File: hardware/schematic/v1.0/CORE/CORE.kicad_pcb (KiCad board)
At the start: 4 copper layers, 0 parts

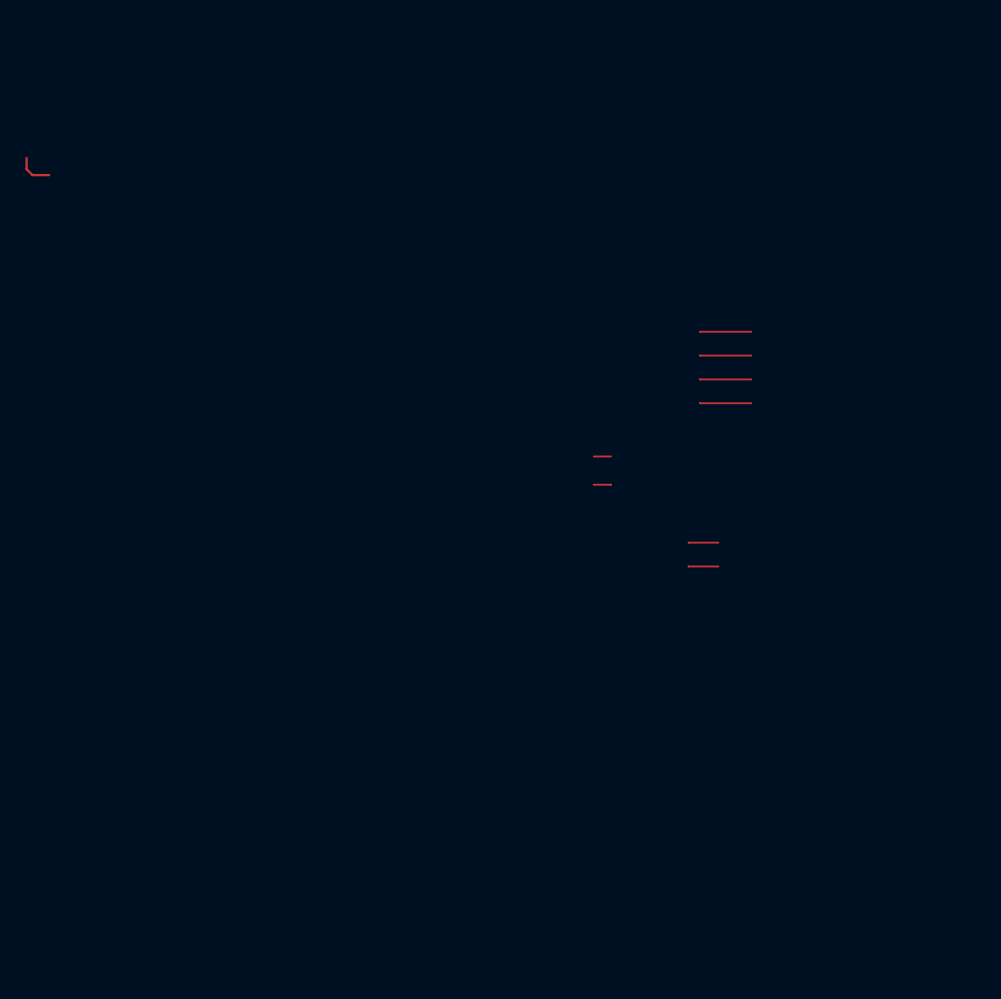
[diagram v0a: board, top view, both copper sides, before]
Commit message: sch and pcb update
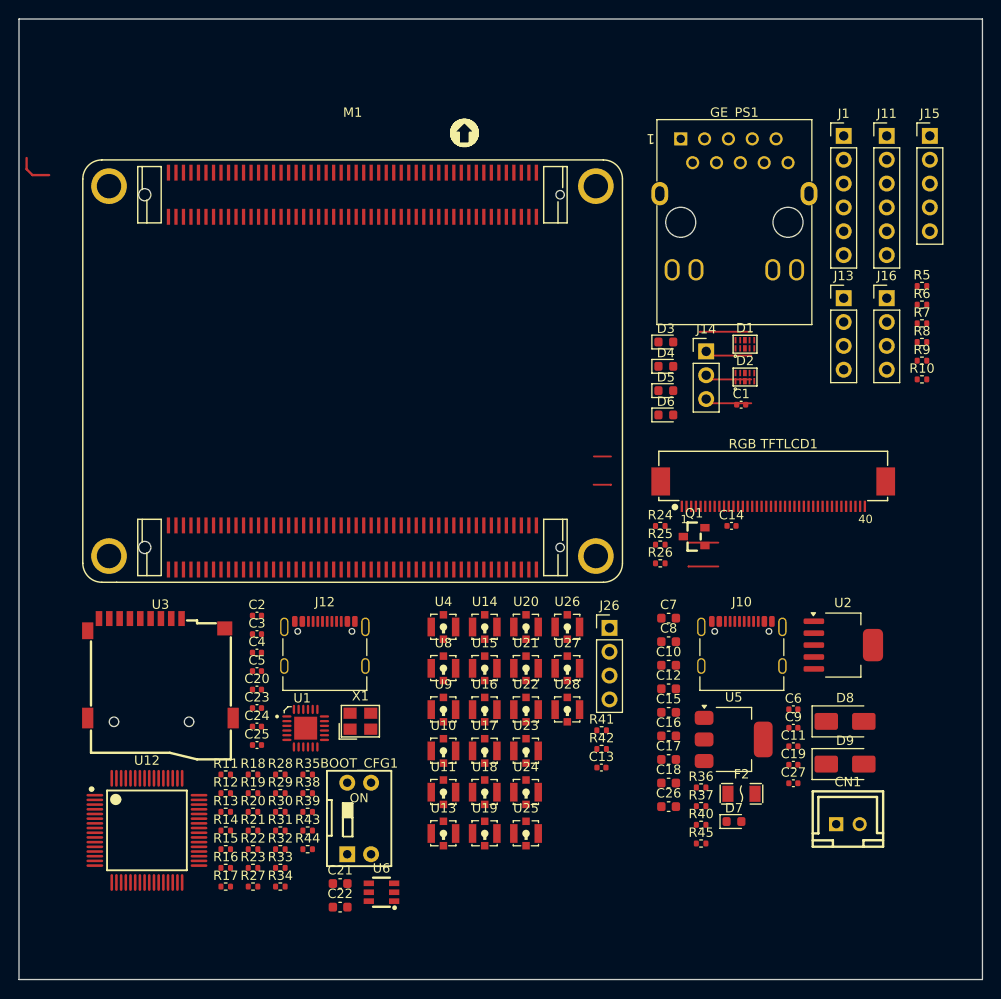
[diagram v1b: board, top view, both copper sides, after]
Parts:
- added BOOT_CFG1: CSW-2P, Counter:CSW DIP-2P, F.Cu at (140.1, 137.9)
- added C1: 100nF, Capacitor_SMD:C_0402_1005Metric, F.Cu at (182.1, 90.0)
- added C10: 10uF, Capacitor_SMD:C_0603_1608Metric, F.Cu at (174.4, 117.7)
- added C11: 100nF, Capacitor_SMD:C_0402_1005Metric, F.Cu at (187.6, 126.4)
- added C12: 10uF, Capacitor_SMD:C_0603_1608Metric, F.Cu at (174.4, 120.3)
- added C13: 1nF, Capacitor_SMD:C_0402_1005Metric, F.Cu at (167.2, 128.6)
- added C14: 100nF, Capacitor_SMD:C_0402_1005Metric, F.Cu at (181.1, 102.9)
- added C15: 10uF, Capacitor_SMD:C_0603_1608Metric, F.Cu at (174.4, 122.8)
- added C16: 100nF, Capacitor_SMD:C_0603_1608Metric, F.Cu at (174.4, 125.3)
- added C17: 10uF, Capacitor_SMD:C_0603_1608Metric, F.Cu at (174.4, 127.8)
- added C18: 100nF, Capacitor_SMD:C_0603_1608Metric, F.Cu at (174.4, 130.3)
- added C19: 100nF, Capacitor_SMD:C_0402_1005Metric, F.Cu at (187.6, 128.3)
- added C2: 100nF, Capacitor_SMD:C_0402_1005Metric, F.Cu at (130.5, 112.5)
- added C20: 100nF, Capacitor_SMD:C_0402_1005Metric, F.Cu at (130.5, 120.3)
- added C21: 10uF, Capacitor_SMD:C_0603_1608Metric, F.Cu at (139.4, 141.0)
- added C22: 10uF, Capacitor_SMD:C_0603_1608Metric, F.Cu at (139.4, 143.5)
- added C23: 100nF, Capacitor_SMD:C_0402_1005Metric, F.Cu at (130.5, 122.3)
- added C24: 30pF, Capacitor_SMD:C_0402_1005Metric, F.Cu at (130.5, 124.3)
- added C25: 30pF, Capacitor_SMD:C_0402_1005Metric, F.Cu at (130.5, 126.2)
- added C26: 10uF, Capacitor_SMD:C_0603_1608Metric, F.Cu at (174.4, 132.8)
- added C27: 100nF, Capacitor_SMD:C_0402_1005Metric, F.Cu at (187.6, 130.3)
- added C3: 100nF, Capacitor_SMD:C_0402_1005Metric, F.Cu at (130.5, 114.4)
- added C4: 10uF, Capacitor_SMD:C_0402_1005Metric, F.Cu at (130.5, 116.4)
- added C5: 100nF, Capacitor_SMD:C_0402_1005Metric, F.Cu at (130.5, 118.4)
- added C6: 100nF, Capacitor_SMD:C_0402_1005Metric, F.Cu at (187.6, 122.4)
- added C7: 10uF, Capacitor_SMD:C_0603_1608Metric, F.Cu at (174.4, 112.7)
- added C8: 10uF, Capacitor_SMD:C_0603_1608Metric, F.Cu at (174.4, 115.2)
- added C9: 10nF, Capacitor_SMD:C_0402_1005Metric, F.Cu at (187.6, 124.4)
- added CN1: LAIL-PHC2_54-2P-01-XH-L, JLCImport:LAIL-PHC2_54-2P-01-XH-L, F.Cu at (193.5, 134.7)
- added D1: AZ1143-04F.R7G, Counter:DFN2510P10E, F.Cu at (181.4, 84.8)
- added D2: AZ1143-04F.R7G, Counter:DFN2510P10E, F.Cu at (181.4, 88.3)
- added D3: LED, LED_SMD:LED_0603_1608Metric, F.Cu at (174.1, 83.3)
- added D4: LED, LED_SMD:LED_0603_1608Metric, F.Cu at (174.1, 85.9)
- added D5: LED, LED_SMD:LED_0603_1608Metric, F.Cu at (174.1, 88.5)
- added D6: LED, LED_SMD:LED_0603_1608Metric, F.Cu at (174.1, 91.1)
- added D7: LED, LED_SMD:LED_0603_1608Metric, F.Cu at (181.3, 134.4)
- added D8: SS34, Diode_SMD:D_SMA, F.Cu at (193.2, 123.7)
- added D9: SS34, Diode_SMD:D_SMA, F.Cu at (193.2, 128.3)
- added F2: BSMD1206C-1300T, JLCImport:BSMD1206C-1300T, F.Cu at (182.1, 131.4)
- added GE_PS1: HR911131A, Counter:HR911131A, F.Cu at (175.6, 61.7)
- added J1: Conn_01x06_Socket, Connector_PinHeader_2.54mm:PinHeader_1x06_P2.54mm_Vertical, F.Cu at (193.0, 61.3)
- added J10: USB_C_Receptacle_USB2.0_16P, Connector_USB:USB_C_Receptacle_Palconn_UTC16-G, F.Cu at (182.2, 115.6)
- added J11: Conn_01x06_Socket, Connector_PinHeader_2.54mm:PinHeader_1x06_P2.54mm_Vertical, F.Cu at (197.6, 61.3)
- added J12: USB_C_Receptacle_USB2.0_16P, Connector_USB:USB_C_Receptacle_Palconn_UTC16-G, F.Cu at (137.7, 115.6)
- added J13: Conn_01x04_Socket, Connector_PinHeader_2.54mm:PinHeader_1x04_P2.54mm_Vertical, F.Cu at (193.0, 78.6)
- added J14: Conn_01x03_Socket, Connector_PinHeader_2.54mm:PinHeader_1x03_P2.54mm_Vertical, F.Cu at (178.4, 84.3)
- added J15: Conn_01x05_Socket, Connector_PinHeader_2.54mm:PinHeader_1x05_P2.54mm_Vertical, F.Cu at (202.2, 61.3)
- added J16: Conn_01x04_Socket, Connector_PinHeader_2.54mm:PinHeader_1x04_P2.54mm_Vertical, F.Cu at (197.6, 78.6)
- added J26: Conn_01x04_Socket, Connector_PinHeader_2.54mm:PinHeader_1x04_P2.54mm_Vertical, F.Cu at (168.1, 113.8)
- added M1: ZYNQ7010&7020, Counter:ZYNQ7010&7020_CB, F.Cu at (126.3, 102.8)
- added Q1: Si2302CDS-T1-GE3, JLCImport:Si2302CDS-T1-GE3, F.Cu at (177.1, 104.0)
- added R10: 499R, Resistor_SMD:R_0402_1005Metric, F.Cu at (201.3, 87.3)
- added R11: 20K, Resistor_SMD:R_0402_1005Metric, F.Cu at (127.2, 129.4)
- added R12: 20K, Resistor_SMD:R_0402_1005Metric, F.Cu at (127.2, 131.4)
- added R13: 10K, Resistor_SMD:R_0402_1005Metric, F.Cu at (127.2, 133.4)
- added R14: 10K, Resistor_SMD:R_0402_1005Metric, F.Cu at (127.2, 135.4)
- added R15: 4.7K, Resistor_SMD:R_0402_1005Metric, F.Cu at (127.2, 137.3)
- added R16: 330, Resistor_SMD:R_0402_1005Metric, F.Cu at (127.2, 139.3)
- added R17: 0, Resistor_SMD:R_0402_1005Metric, F.Cu at (127.2, 141.3)
- added R18: 10K, Resistor_SMD:R_0402_1005Metric, F.Cu at (130.1, 129.4)
- added R19: 4.7K, Resistor_SMD:R_0402_1005Metric, F.Cu at (130.1, 131.4)
- added R20: 4.7K, Resistor_SMD:R_0402_1005Metric, F.Cu at (130.1, 133.4)
- added R21: 4.7K, Resistor_SMD:R_0402_1005Metric, F.Cu at (130.1, 135.4)
- added R22: 4.7K, Resistor_SMD:R_0402_1005Metric, F.Cu at (130.1, 137.3)
- added R23: 4.7K, Resistor_SMD:R_0402_1005Metric, F.Cu at (130.1, 139.3)
- added R24: 10K, Resistor_SMD:R_0402_1005Metric, F.Cu at (173.5, 102.9)
- added R25: 1K, Resistor_SMD:R_0402_1005Metric, F.Cu at (173.5, 104.9)
- added R26: 10, Resistor_SMD:R_0402_1005Metric, F.Cu at (173.5, 106.9)
- added R27: 10R, Resistor_SMD:R_0402_1005Metric, F.Cu at (130.1, 141.3)
- added R28: 10R, Resistor_SMD:R_0402_1005Metric, F.Cu at (133.0, 129.4)
- added R29: 33R, Resistor_SMD:R_0402_1005Metric, F.Cu at (133.0, 131.4)
- added R30: 33R, Resistor_SMD:R_0402_1005Metric, F.Cu at (133.0, 133.4)
- added R31: 33R, Resistor_SMD:R_0402_1005Metric, F.Cu at (133.0, 135.4)
- added R32: 33R, Resistor_SMD:R_0402_1005Metric, F.Cu at (133.0, 137.3)
- added R33: 2K, Resistor_SMD:R_0402_1005Metric, F.Cu at (133.0, 139.3)
- added R34: 10K, Resistor_SMD:R_0402_1005Metric, F.Cu at (133.0, 141.3)
- added R35: 12K/%1, Resistor_SMD:R_0402_1005Metric, F.Cu at (135.9, 129.4)
- added R36: 5.1K, Resistor_SMD:R_0402_1005Metric, F.Cu at (177.8, 130.8)
- added R37: 5.1K, Resistor_SMD:R_0402_1005Metric, F.Cu at (177.8, 132.8)
- added R38: 5.1K, Resistor_SMD:R_0402_1005Metric, F.Cu at (135.9, 131.4)
- added R39: 5.1K, Resistor_SMD:R_0402_1005Metric, F.Cu at (135.9, 133.4)
- added R40: 0, Resistor_SMD:R_0402_1005Metric, F.Cu at (177.8, 134.7)
- added R41: 49.9, Resistor_SMD:R_0402_1005Metric, F.Cu at (167.2, 124.7)
- added R42: 49.9, Resistor_SMD:R_0402_1005Metric, F.Cu at (167.2, 126.7)
- added R43: 0, Resistor_SMD:R_0402_1005Metric, F.Cu at (135.9, 135.4)
- added R44: 0, Resistor_SMD:R_0402_1005Metric, F.Cu at (135.9, 137.3)
- added R45: 1K, Resistor_SMD:R_0402_1005Metric, F.Cu at (177.8, 136.7)
- added R5: 499R, Resistor_SMD:R_0402_1005Metric, F.Cu at (201.3, 77.3)
- added R6: 499R, Resistor_SMD:R_0402_1005Metric, F.Cu at (201.3, 79.3)
- added R7: 499R, Resistor_SMD:R_0402_1005Metric, F.Cu at (201.3, 81.3)
- added R8: 499R, Resistor_SMD:R_0402_1005Metric, F.Cu at (201.3, 83.3)
- added R9: 499R, Resistor_SMD:R_0402_1005Metric, F.Cu at (201.3, 85.3)
- added RGB TFTLCD1: RGBLCD, AD:FPC-TOP40, F.Cu at (175.8, 100.9)
- added U1: TXS02612RTWR, Counter:QFN24_RTW, F.Cu at (135.7, 124.4)
- added U10: IPEX1, Counter:JLC_IPEX-1, F.Cu at (150.4, 126.9)
- added U11: IPEX1, Counter:JLC_IPEX-1, F.Cu at (150.4, 131.3)
- added U12: FT2232HL, JLCImport:FT2232HL, F.Cu at (118.8, 135.3)
- added U13: IPEX1, Counter:JLC_IPEX-1, F.Cu at (150.4, 135.7)
- added U14: IPEX1, Counter:JLC_IPEX-1, F.Cu at (154.8, 113.7)
- added U15: IPEX1, Counter:JLC_IPEX-1, F.Cu at (154.8, 118.1)
- added U16: IPEX1, Counter:JLC_IPEX-1, F.Cu at (154.8, 122.5)
- added U17: IPEX1, Counter:JLC_IPEX-1, F.Cu at (154.8, 126.9)
- added U18: IPEX1, Counter:JLC_IPEX-1, F.Cu at (154.8, 131.3)
- added U19: IPEX1, Counter:JLC_IPEX-1, F.Cu at (154.8, 135.7)
- added U2: TPS78633, Package_TO_SOT_SMD:SOT-223-6, F.Cu at (193.0, 115.6)
- added U20: IPEX1, Counter:JLC_IPEX-1, F.Cu at (159.2, 113.7)
- added U21: IPEX1, Counter:JLC_IPEX-1, F.Cu at (159.2, 118.1)
- added U22: IPEX1, Counter:JLC_IPEX-1, F.Cu at (159.2, 122.5)
- added U23: IPEX1, Counter:JLC_IPEX-1, F.Cu at (159.2, 126.9)
- added U24: IPEX1, Counter:JLC_IPEX-1, F.Cu at (159.2, 131.3)
- added U25: IPEX1, Counter:JLC_IPEX-1, F.Cu at (159.2, 135.7)
- added U26: IPEX1, Counter:JLC_IPEX-1, F.Cu at (163.6, 113.7)
- added U27: IPEX1, Counter:JLC_IPEX-1, F.Cu at (163.6, 118.1)
- added U28: IPEX1, Counter:JLC_IPEX-1, F.Cu at (163.6, 122.5)
- added U3: SD_Card, Counter:SIM-SMD_LX_XDFP-0090-012, F.Cu at (120.2, 118.1)
- added U4: IPEX1, Counter:JLC_IPEX-1, F.Cu at (150.4, 113.7)
- added U5: AMS1117-1.8, Package_TO_SOT_SMD:SOT-223-3_TabPin2, F.Cu at (181.3, 125.7)
- added U6: 93LC56BT-I_OT, JLCImport:93LC56BT-I_OT, F.Cu at (143.8, 141.9)
- added U8: IPEX1, Counter:JLC_IPEX-1, F.Cu at (150.4, 118.1)
- added U9: IPEX1, Counter:JLC_IPEX-1, F.Cu at (150.4, 122.5)
- added X1: X322512MSB4SI, JLCImport:X322512MSB4SI, F.Cu at (141.5, 123.7)
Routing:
- net (no net): track 0.00 -> 16.4 mm
- net Net-(JTAG1-Pad10): track 5.47 -> 0.00 mm
- net Net-(JTAG1-Pad8): track 5.47 -> 0.00 mm
- net /Comm_Periph/PS_I2C_SDA: track 0.00 -> 5.47 mm
- net Net-(JTAG1-Pad6): track 5.47 -> 0.00 mm
- net Net-(JTAG1-Pad4): track 5.46 -> 0.00 mm
- net Net-(Q1-G): track 0.00 -> 3.16 mm
- net Net-(BOOT_CFG1-Pad3): track 3.16 -> 0.00 mm
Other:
- board outline added: 102.6 x 102.3 mm
